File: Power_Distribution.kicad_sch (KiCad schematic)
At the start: 27 parts, among them IC3 LP5912-3.3DRVR, J7 CarPowerConnector, Q1 PBSS4330X,135, Q3 SI7149ADP-T1-GE3

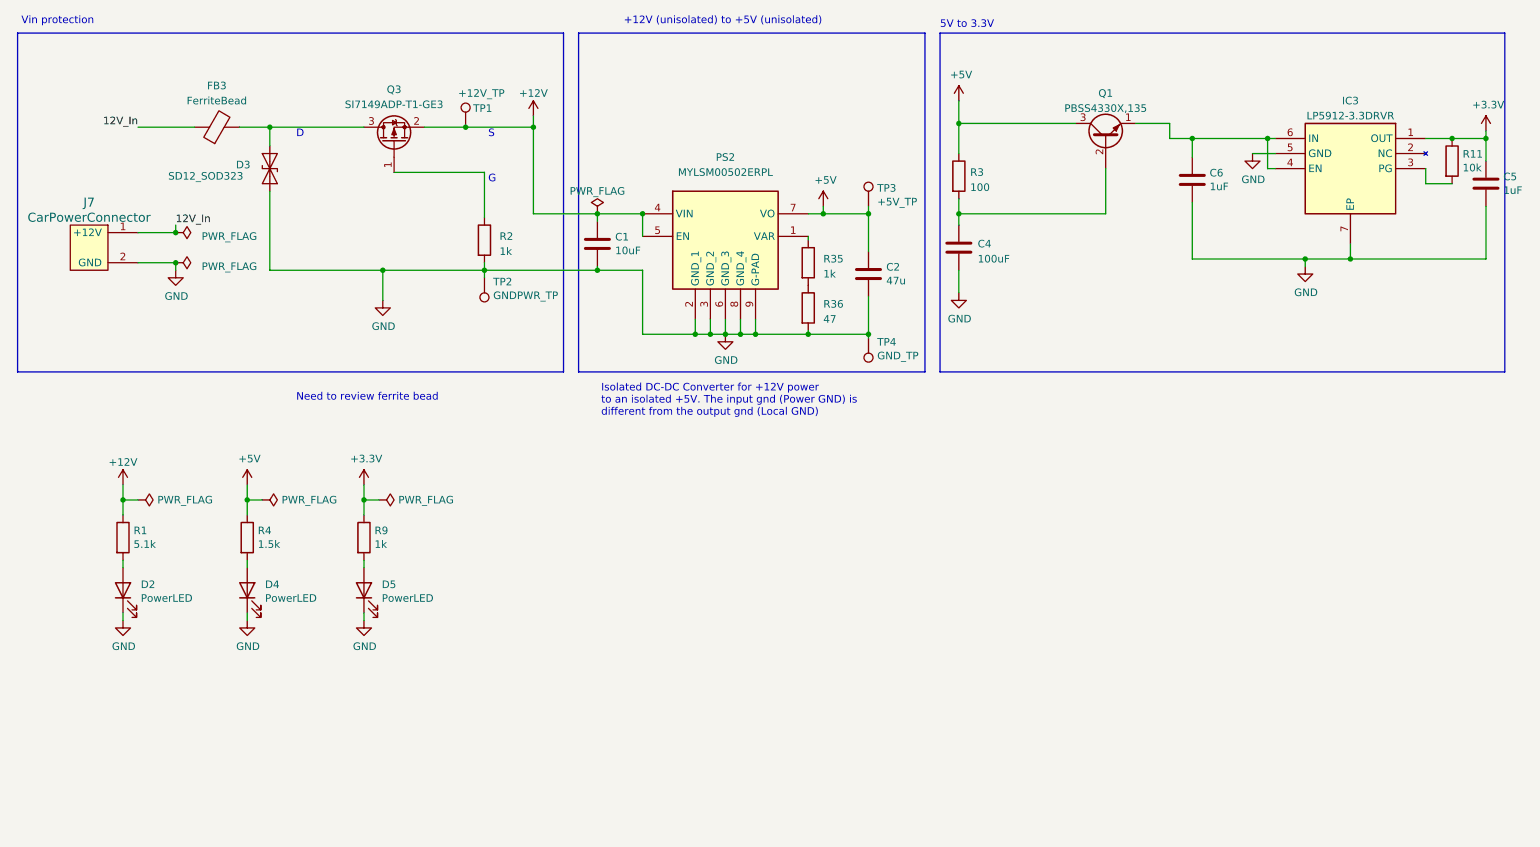
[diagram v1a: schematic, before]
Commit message: a
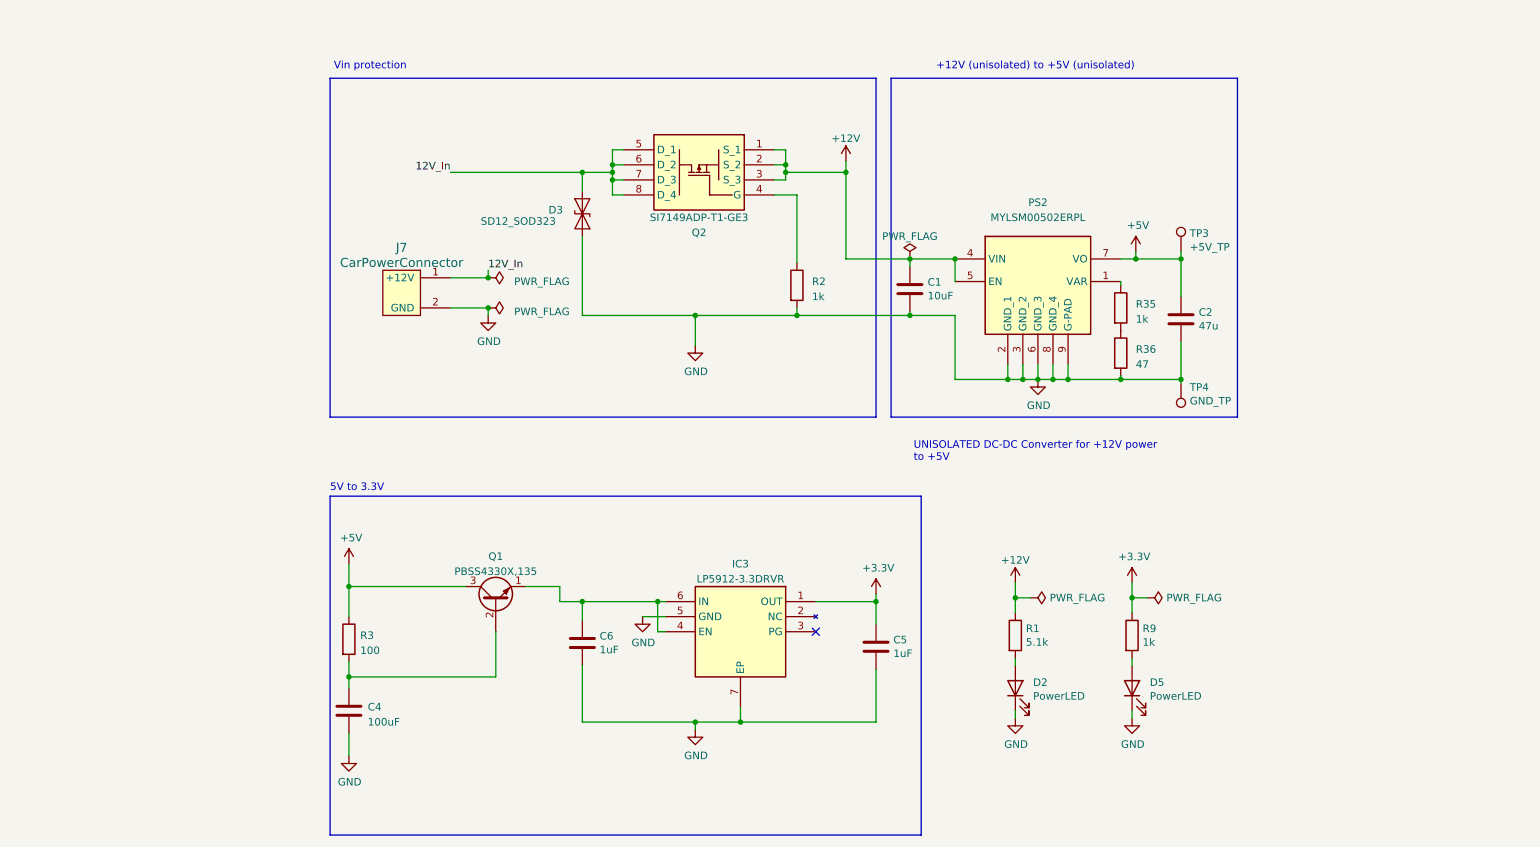
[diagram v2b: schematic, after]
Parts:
- removed D4: PowerLED, LED_SMD:LED_0805_2012Metric, symbol Device:LED
- removed FB3: FerriteBead, Inductor_SMD:L_0805_2012Metric, symbol Device:FerriteBead
- removed Q3: SI7149ADP-T1-GE3, Package_TO_SOT_SMD:SOT-23, symbol Transistor_FET:AO3401A
- removed R11: 10k, Resistor_SMD:R_0805_2012Metric, symbol Device:R
- removed R4: 1.5k, Resistor_SMD:R_0805_2012Metric, symbol Device:R
- removed TP1: +12V_TP, TestPoint:TestPoint_Keystone_5005-5009_Compact, symbol Connector:TestPoint
- removed TP2: GNDPWR_TP, TestPoint:TestPoint_Keystone_5005-5009_Compact, symbol Connector:TestPoint
- added Q2: SI7149ADP-T1-GE3, POWERPAKSO-8, symbol utsvt-chips:SI7149ADP-T1-GE3
- C1: footprint UTSVT_Passive:C_2220_5750Metric -> Capacitor_SMD:C_0805_2012Metric; Mouser Part Number 581-22201C106KAT2A -> 963-TMK212BBJ106MGHT; P/N 22201C106KAT2A -> TMK212BBJ106MGHT
- C2: footprint UTSVT_Passive:C_2220_5750Metric -> Capacitor_SMD:C_0805_2012Metric; Mouser Part Number 581-22201C106KAT2A -> 81-GRM21B80J476ME01K; P/N 22201C106KAT2A -> GRM21BC80J476ME01K
- C4: footprint Capacitor_SMD:C_0805_2012Metric -> Capacitor_SMD:C_1206_3216Metric; Mouser Part Number (none) -> 187-CL31A107MPKNNWE; P/N (none) -> CL31A107MPKNNWE
- PS2: footprint MYLSM00502ERPL -> UTSVT_Power:MYLSM00502ERPL
- Q1: footprint Package_TO_SOT_THT:TO-39-3 -> Package_TO_SOT_SMD:SOT-89-3
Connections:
- net +12V: now also Q2.1 (S_1), Q2.2 (S_2), Q2.3 (S_3)
- net 12V_In: now also D3.2 (A2), Q2.5 (D_1), Q2.6 (D_2), Q2.7 (D_3), Q2.8 (D_4)
- net at R2.1: now also Q2.4 (G)
- no-connect marks 0 -> 1
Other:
- note added: "UNISOLATED DC-DC Converter for +12V power to +5V"
- note removed: "D"
- note removed: "G"
- note removed: "Isolated DC-DC Converter for +12V power to an isolated +5V. The input gnd (Power GND) is different from the output gnd (Local GND)"
- note removed: "Need to review ferrite bead"
- note removed: "S"
- moved on the sheet: C1, C2, C4, C5, C6, D2, D3, D5, IC3, J7, PS2, Q1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
